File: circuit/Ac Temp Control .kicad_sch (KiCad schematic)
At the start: 21 parts, among them J1 USB_B_Micro, Q1 P2N2222A, SW1 SW_Push, SW2 SW_Push, SW3 SW_Push, SW4 SW_Push, U1 AMS1117-5.0, U2 ATmega328-P, U3 DHT11, U4 TSOP382xx, Y1 16MHZ

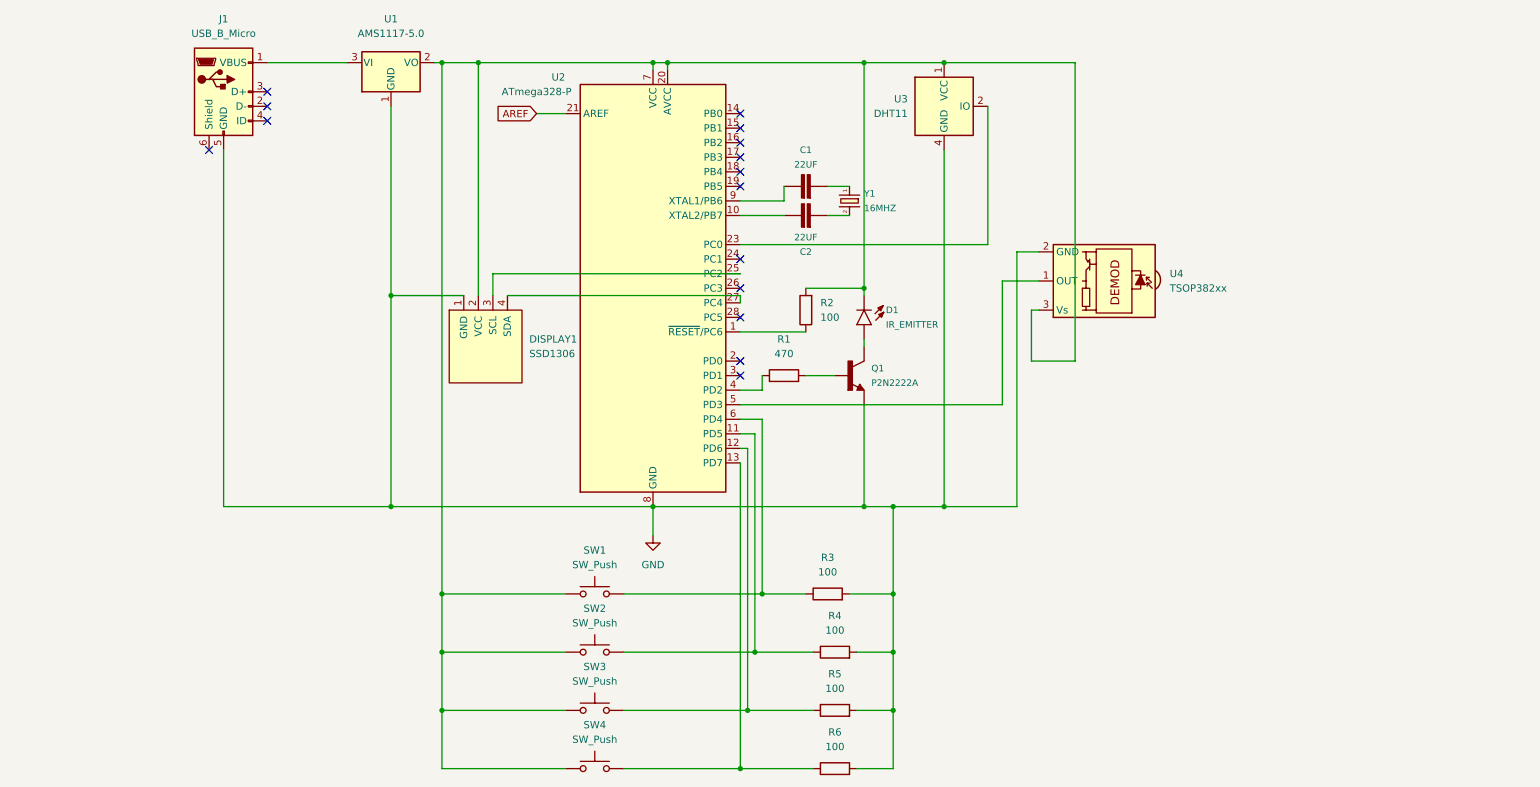
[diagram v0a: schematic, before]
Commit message: Add files via upload
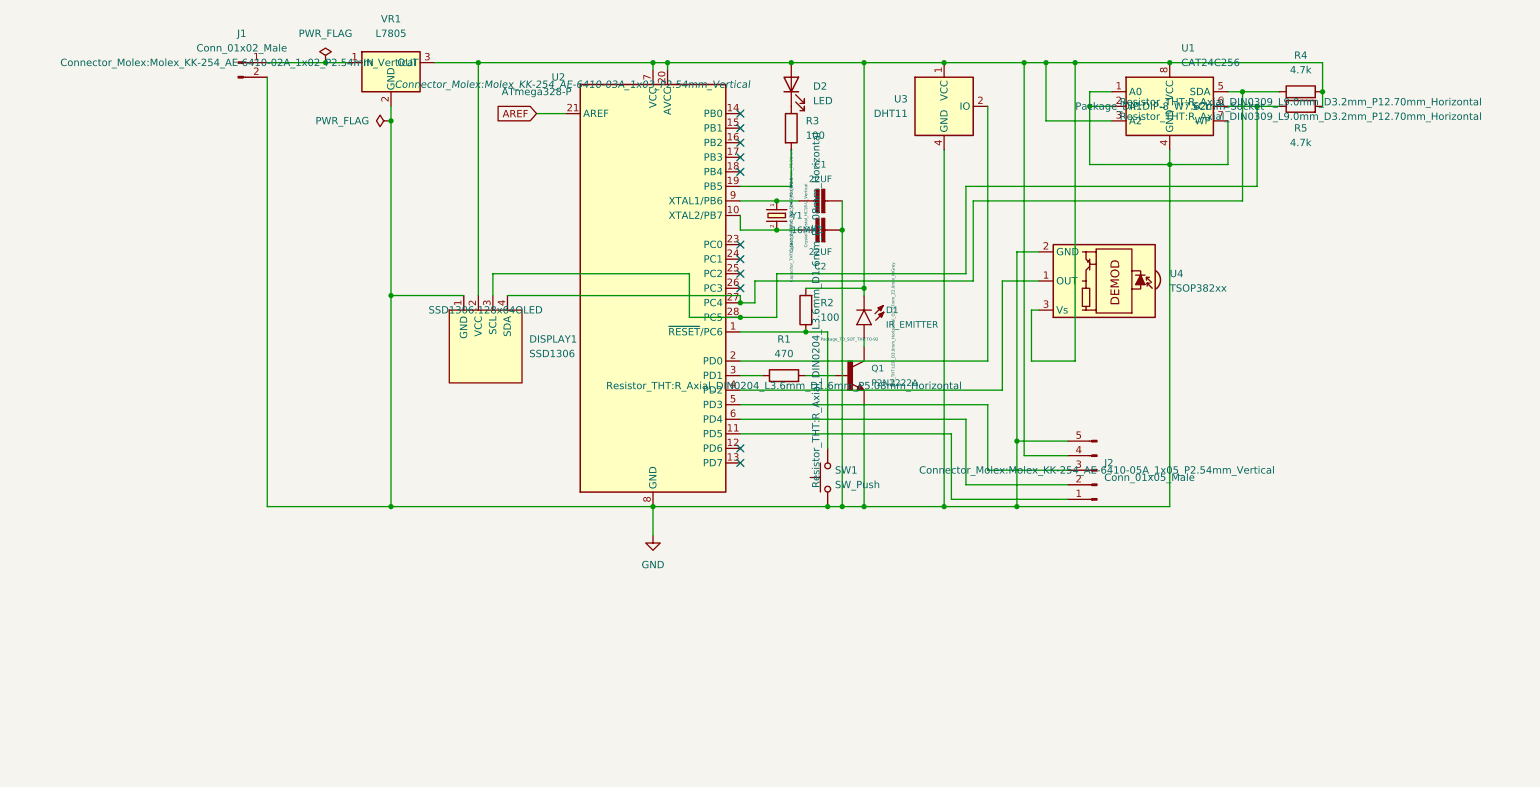
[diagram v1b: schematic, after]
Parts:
- removed J1: USB_B_Micro, Connector_USB:USB_Micro-B_Amphenol_10103594-0001LF_Horizontal, symbol Connector:USB_B_Micro
- removed R6: 100, Resistor_THT:R_Axial_DIN0204_L3.6mm_D1.6mm_P5.08mm_Horizontal, symbol Device:R
- removed SW2, SW3, SW4: SW_Push, Button_Switch_THT:SW_PUSH_6mm, symbol Switch:SW_Push
- removed U1: AMS1117-5.0, Package_TO_SOT_SMD:SOT-223-3_TabPin2, symbol Regulator_Linear:AMS1117-5.0
- added D2: LED, LED_THT:LED_D1.8mm_W1.8mm_H2.4mm_Horizontal_O1.27mm_Z1.6mm, symbol Device:LED
- added J1: Conn_01x02_Male, Connector_Molex:Molex_KK-254_AE-6410-02A_1x02_P2.54mm_Vertical, symbol Connector:Conn_01x02_Male
- added J2: Conn_01x05_Male, Connector_Molex:Molex_KK-254_AE-6410-05A_1x05_P2.54mm_Vertical, symbol Connector:Conn_01x05_Male
- added U1: CAT24C256, Package_DIP:DIP-8_W7.62mm_Socket, symbol Memory_EEPROM:CAT24C256
- added VR1: L7805, Connector_Molex:Molex_KK-254_AE-6410-03A_1x03_P2.54mm_Vertical, symbol Regulator_Linear:L7805
- R3: footprint Resistor_THT:R_Axial_DIN0204_L3.6mm_D1.6mm_P5.08mm_Horizontal -> Resistor_THT:R_Axial_DIN0207_L6.3mm_D2.5mm_P10.16mm_Horizontal
- R4, R5: value 100 -> 4.7k; footprint Resistor_THT:R_Axial_DIN0204_L3.6mm_D1.6mm_P5.08mm_Horizontal -> Resistor_THT:R_Axial_DIN0309_L9.0mm_D3.2mm_P12.70mm_Horizontal
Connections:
- net GND: now also C1.2, C2.2, SW1.1, J1.2 (Pin_2), J2.5 (Pin_5), U1.1 (A0), U1.2 (A1), U1.4 (GND), U1.7 (WP), VR1.2 (GND); no longer R3.2, R4.2, R5.2
- net at D1.C, DISPLAY1.2 (VCC), R2.2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: now also R4.2, R5.2, D2.2 (A), J2.4 (Pin_4), U1.3 (A2), U1.8 (VCC), VR1.3 (OUT); no longer SW1.1
- net at DISPLAY1.3 (SCL): now also R5.1, U2.28 (PC5), U1.6 (SCL); no longer U2.25 (PC2)
- net at DISPLAY1.4 (SDA), U2.27 (PC4): now also R4.1, U1.5 (SDA)
- net at U3.2 (IO): now also U2.2 (PD0); no longer U2.23 (PC0)
- net at U2.11 (PD5): now also J2.1 (Pin_1); no longer R4.1
- net at R2.1, U2.1 (~{RESET}/PC6): now also SW1.2
- net at C1.1, U2.9 (XTAL1/PB6): now also Y1.1
- net at U2.12 (PD6): no longer R5.1
- net at Y1.2: now also C2.1, U2.10 (XTAL2/PB7); no longer C2.2
- net at R1.1: now also U2.3 (PD1); no longer U2.4 (PD2)
- net at U2.19 (PB5): now also R3.2
- net at U2.5 (PD3): now also J2.3 (Pin_3); no longer U4.1 (OUT)
- new net: D2.1 (K), R3.1
- new net: J2.2 (Pin_2), U2.6 (PD4)
- new net: J1.1 (Pin_1), VR1.1 (IN)
- new net: U2.4 (PD2), U4.1 (OUT)
- no-connect marks 15 -> 11
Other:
- moved on the sheet: C1, C2, Y1

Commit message: PCB design and Gerber file generation
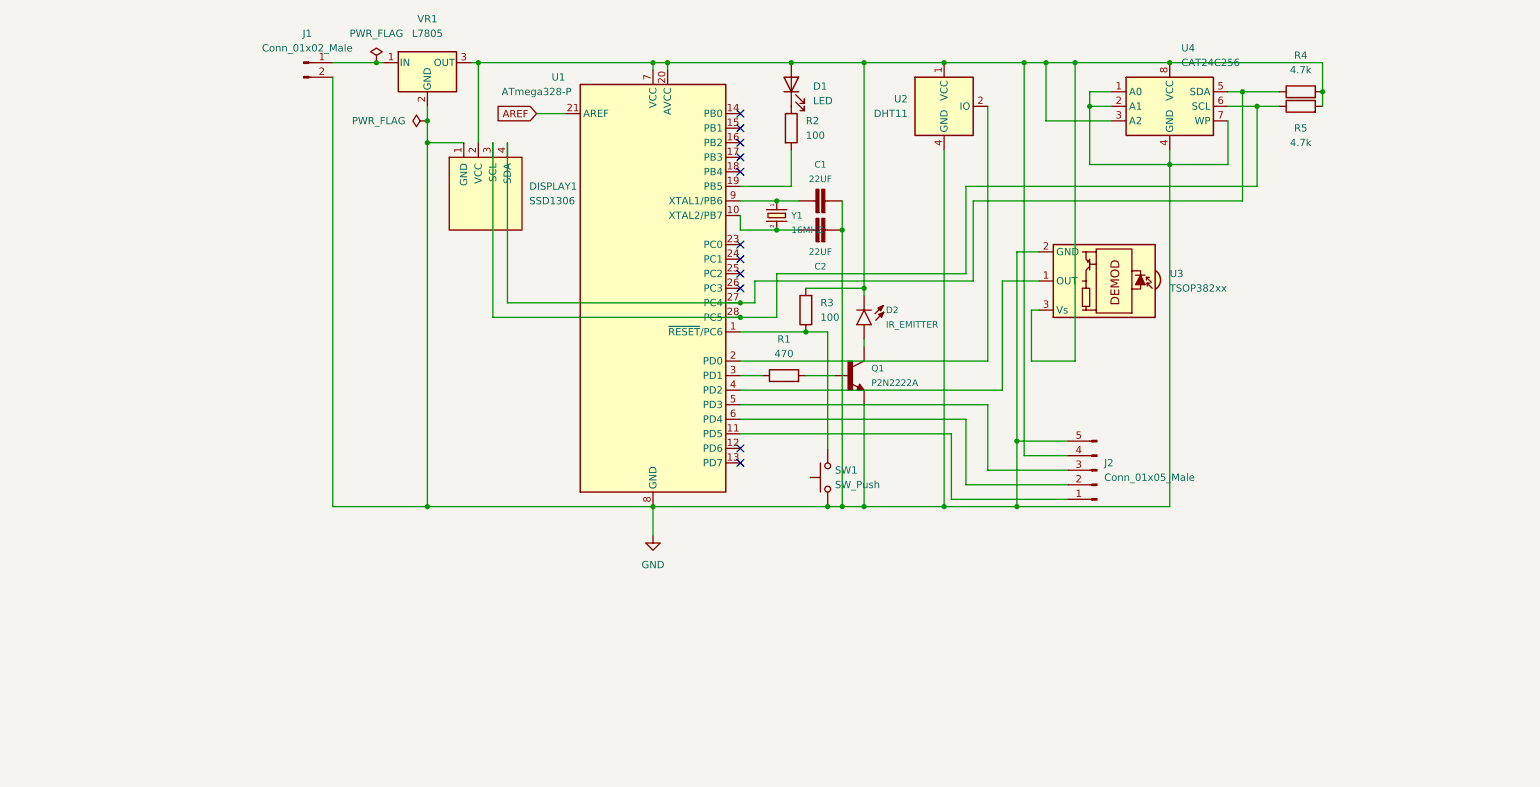
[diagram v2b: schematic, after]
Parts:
- D1: renamed from D2; footprint LED_THT:LED_D1.8mm_W1.8mm_H2.4mm_Horizontal_O1.27mm_Z1.6mm -> LED_THT:LED_D3.0mm_Horizontal_O1.27mm_Z10.0mm
- D2: renamed from D1; footprint LED_THT:LED_D3.0mm_Horizontal_O1.27mm_Z2.0mm_IRGrey -> LED_THT:LED_D5.0mm
- DISPLAY1: footprint SSD1306:128x64OLED -> Connector_Molex:Molex_KK-254_AE-6410-04A_1x04_P2.54mm_Vertical
- R1: footprint Resistor_THT:R_Axial_DIN0204_L3.6mm_D1.6mm_P5.08mm_Horizontal -> Resistor_THT:R_Axial_DIN0207_L6.3mm_D2.5mm_P10.16mm_Horizontal
- R3: renamed from R2; footprint Resistor_THT:R_Axial_DIN0204_L3.6mm_D1.6mm_P5.08mm_Horizontal -> Resistor_THT:R_Axial_DIN0207_L6.3mm_D2.5mm_P10.16mm_Horizontal
- R4, R5: footprint Resistor_THT:R_Axial_DIN0309_L9.0mm_D3.2mm_P12.70mm_Horizontal -> Resistor_THT:R_Axial_DIN0207_L6.3mm_D2.5mm_P10.16mm_Horizontal
- renumbered R3 to R2, U2 to U1, U3 to U2, U4 to U3, U1 to U4
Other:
- moved on the sheet: DISPLAY1, J1, VR1
